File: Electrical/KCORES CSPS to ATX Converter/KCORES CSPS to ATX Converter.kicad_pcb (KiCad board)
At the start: 2 copper layers, 86.1 x 86.1 mm, 29 parts, among them J1 CSPS, J2 PMBUS, J3 GW_PCIe/CPU, J4 GW_PCIe/CPU, J5 GW_PCIe/CPU, J6 GW_PCIe/CPU, J7 GW_PCIe/CPU, J8 IDE/SATA, J9 GW_24P_ATX, U1 PW22 5V, U2 PW22 3.3V, U3 PW22 5V, U4 TPS3511

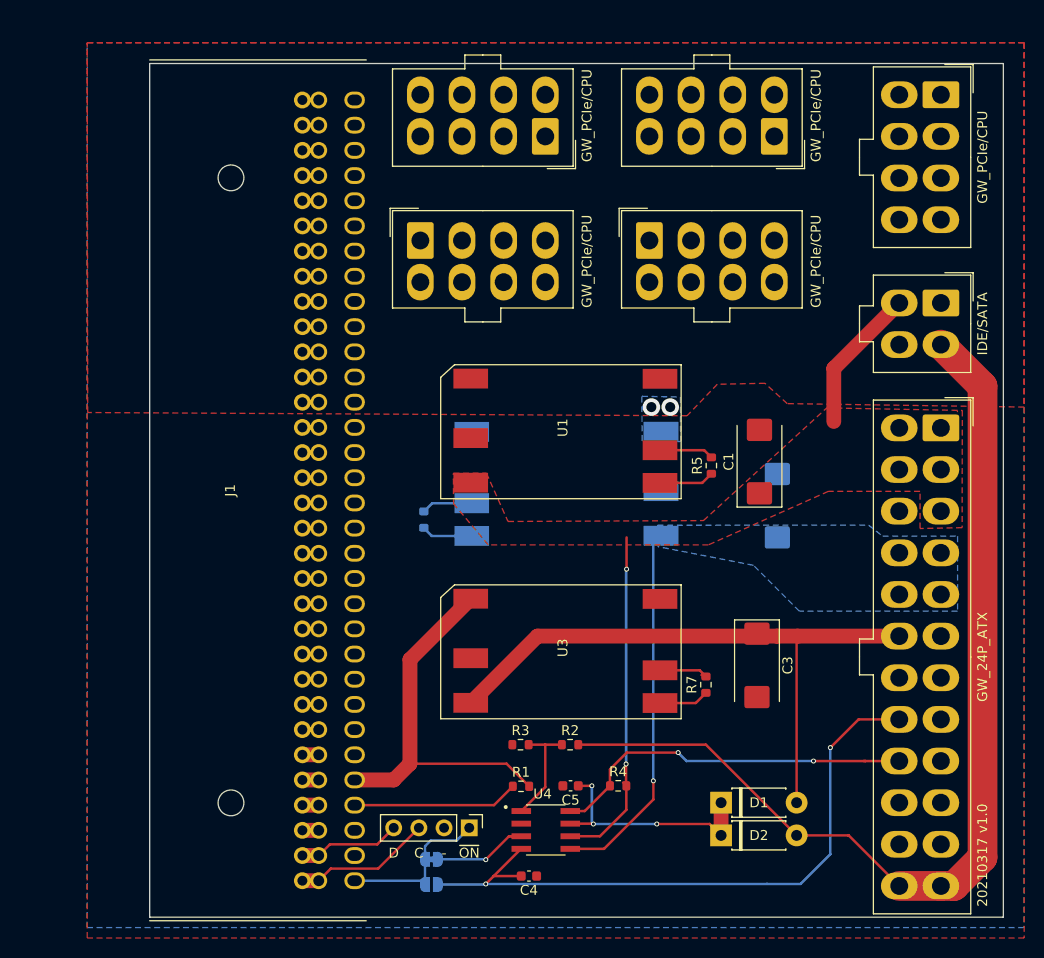
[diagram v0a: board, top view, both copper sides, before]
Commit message: csps part
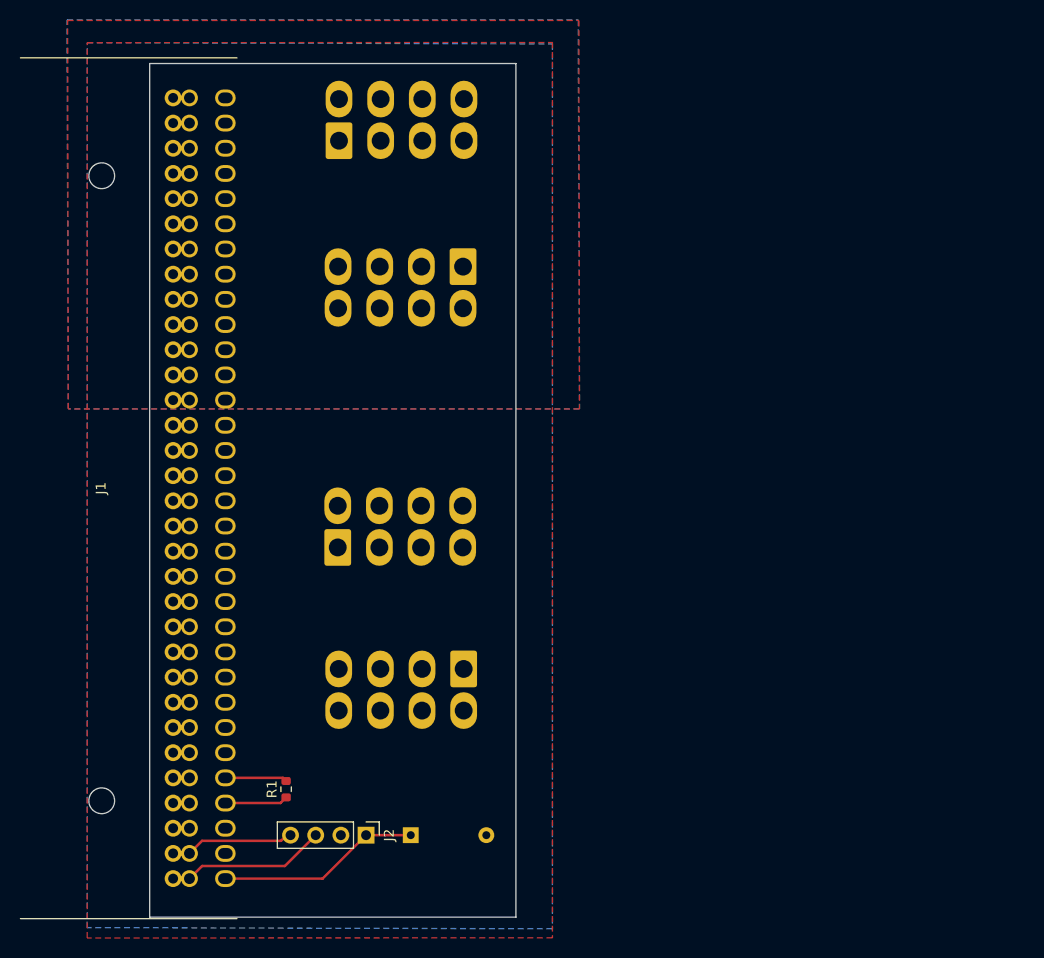
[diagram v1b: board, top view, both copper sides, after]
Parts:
- removed C1, C2, C3: 100uF, Capacitor_Tantalum_SMD:CP_EIA-7343-31_Kemet-D_Pad2.25x2.55mm_HandSolder
- removed C4, C5: 100nF, Capacitor_SMD:C_0603_1608Metric
- removed D1, D2: 1N4001, Diode_THT:D_DO-41_SOD81_P7.62mm_Horizontal
- removed J7: GW_PCIe/CPU, KCORES_Connector_ATX_Power:ATX_8Pin_P4.20mm_Vertical_4.20mm
- removed J8: IDE/SATA, KCORES_Connector_ATX_Power:ATX_4Pin_P4.20mm_Vertical_4.20mm
- removed J9: GW_24P_ATX, KCORES_Connector_ATX_Power:ATX_24Pin_P4.20mm_Vertical_4.20mm
- removed JP1: FPO-CSPS_PSON, Jumper:SolderJumper-2_P1.3mm_Bridged_RoundedPad1.0x1.5mm
- removed JP2: ATX_PSON-CSPS_PSON, Jumper:SolderJumper-2_P1.3mm_Open_RoundedPad1.0x1.5mm
- removed R2: 22K, Resistor_SMD:R_0603_1608Metric
- removed R3, R4: 3.3K, Resistor_SMD:R_0603_1608Metric
- removed R5, R6, R7: R, Resistor_SMD:R_0603_1608Metric
- removed U1, U3: PW22 5V, KCORES_Converter_DCDC:PW22
- removed U2: PW22 3.3V, KCORES_Converter_DCDC:PW22
- removed U4: TPS3511, KCORES_Converter_DCDC:SOIC127P599X175-8N
- added SW1: SW_DIP_x01, Button_Switch_THT:SW_DIP_SPSTx01_Slide_9.78x4.72mm_W7.62mm_P2.54mm, B.Cu at (118.7, 154.5)
- J3, J4, J5, J6: moved to B.Cu
- moved J6 44.1 mm to (111.4, 125.5)
- moved J5 43.9 mm to (111.5, 84.4), turned to 0 degrees
- moved J4 43.4 mm to (124.1, 137.7), turned to 180 degrees
- moved R1 23.7 mm to (106.2, 149.8), turned to 90 degrees
- moved J3 15.5 mm to (124.0, 97.1)
- moved J1 13.0 mm to (79.4, 119.5)
- moved J2 10.4 mm to (114.2, 154.5)
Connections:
- net /CSPS_PSOK renamed Net-(J1-Pad35)
- J3 pad 5: GND -> +12V
- J3 pad 6: GND -> +12V
- J3 pad 7: GND -> +12V
- J3 pad 8: GND -> +12V
- J4 pad 1: +12V -> GND
- J4 pad 2: +12V -> GND
- J4 pad 3: +12V -> GND
- J4 pad 4: +12V -> GND
- J5 pad 5: GND -> +12V
- J5 pad 6: GND -> +12V
- J5 pad 7: GND -> +12V
- J5 pad 8: GND -> +12V
- J6 pad 1: +12V -> GND
- J6 pad 2: +12V -> GND
- J6 pad 3: +12V -> GND
- J6 pad 4: +12V -> GND
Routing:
- net +12V: track 101.5 -> 0.00 mm, vias 2 -> 0
- net /~ATX_PSON: track 67.5 -> 0.00 mm, vias 2 -> 0
- net /+5VSB: track 62.8 -> 0.00 mm
- net +5V: track 49.6 -> 0.00 mm, vias 2 -> 0
- net +3V3: track 37.4 -> 0.00 mm, vias 1 -> 0
- net /ATX_PWOK: track 37.2 -> 0.00 mm, vias 2 -> 0
- net /+12VSB: track 38.4 -> 6.26 mm
- net Net-(C5-Pad1): track 24.2 -> 0.00 mm, vias 3 -> 0
- net Net-(R2-Pad1): track 11.0 -> 0.00 mm
- net /~FPO: track 10.5 -> 0.00 mm, vias 1 -> 0
- net /~PRESENT: track 16.7 -> 6.36 mm
- net Net-(R5-Pad1): track 5.56 -> 0.00 mm
- net Net-(R5-Pad2): track 5.48 -> 0.00 mm
- net Net-(R7-Pad2): track 5.39 -> 0.00 mm
- net Net-(R6-Pad2): track 5.18 -> 0.00 mm
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- removed copper zone on B.Cu, net +3V3
- removed copper zone on F.Cu, net +5V
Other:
- board size 86.1 x 86.1 mm -> 36.9 x 86.1 mm
- board text removed: "-"
- board text removed: "20210317 v1.0"
- board text removed: "C"
- board text removed: "CSPS to ATX Converter"
- board text removed: "Contributor: AlphaArea Ubiq"
- board text removed: "D"
- board text removed: "KCORES"
- board text removed: "~ON"
